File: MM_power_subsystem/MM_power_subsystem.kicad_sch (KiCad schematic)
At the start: 0 parts

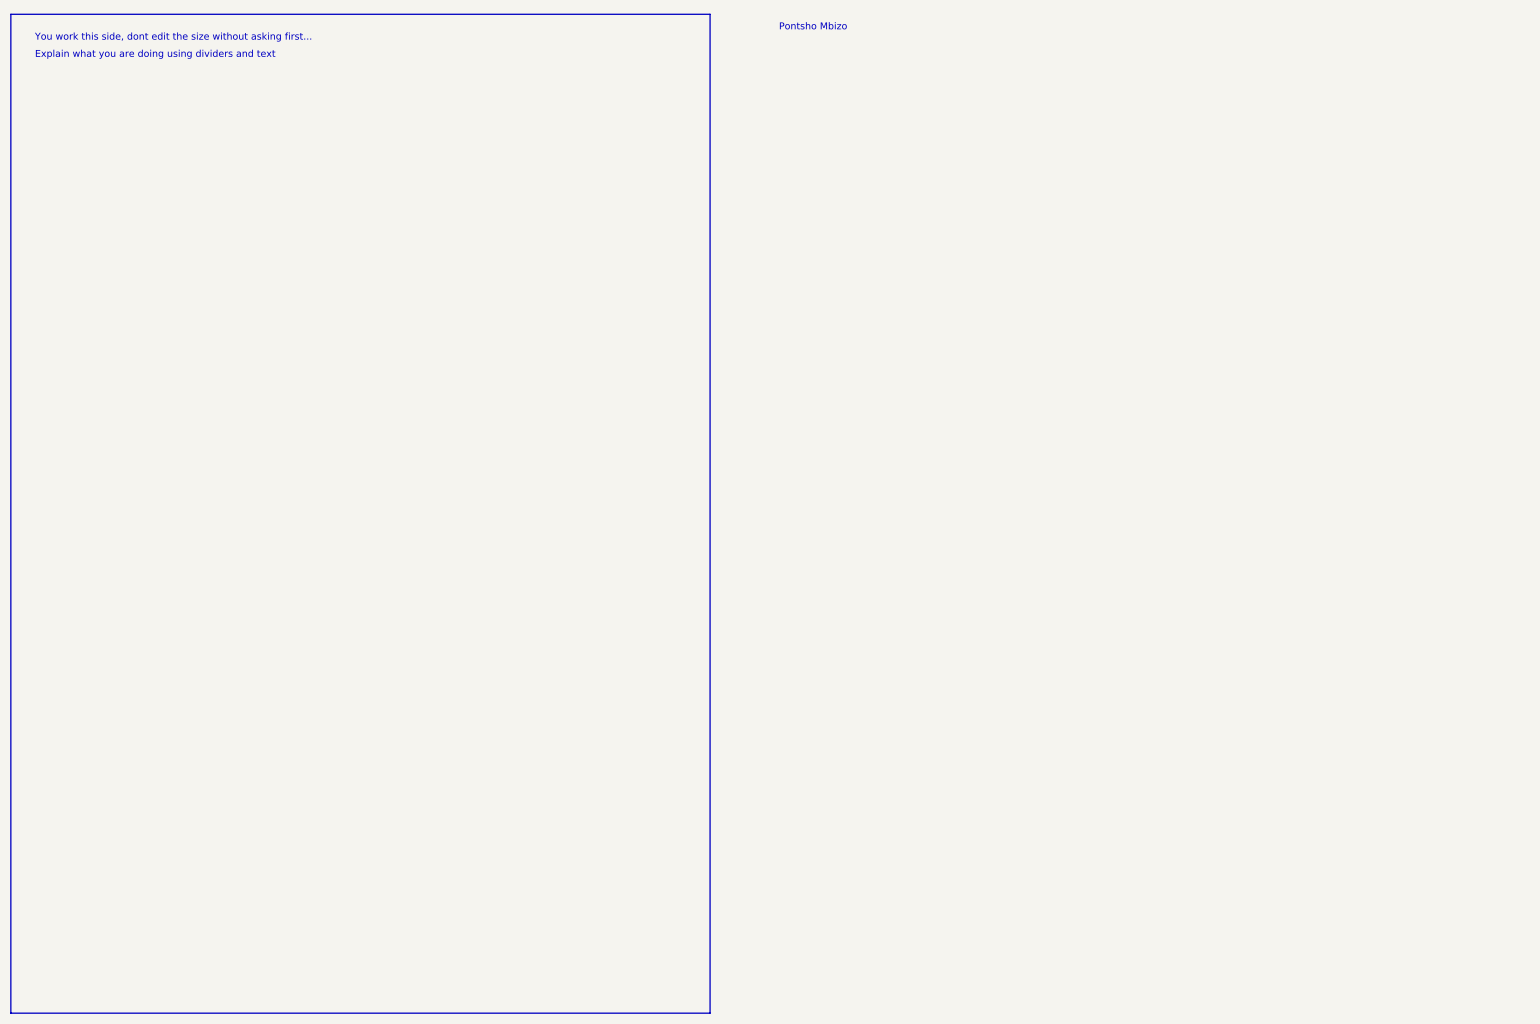
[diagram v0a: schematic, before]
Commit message: Done with the first version of my subsub systems.
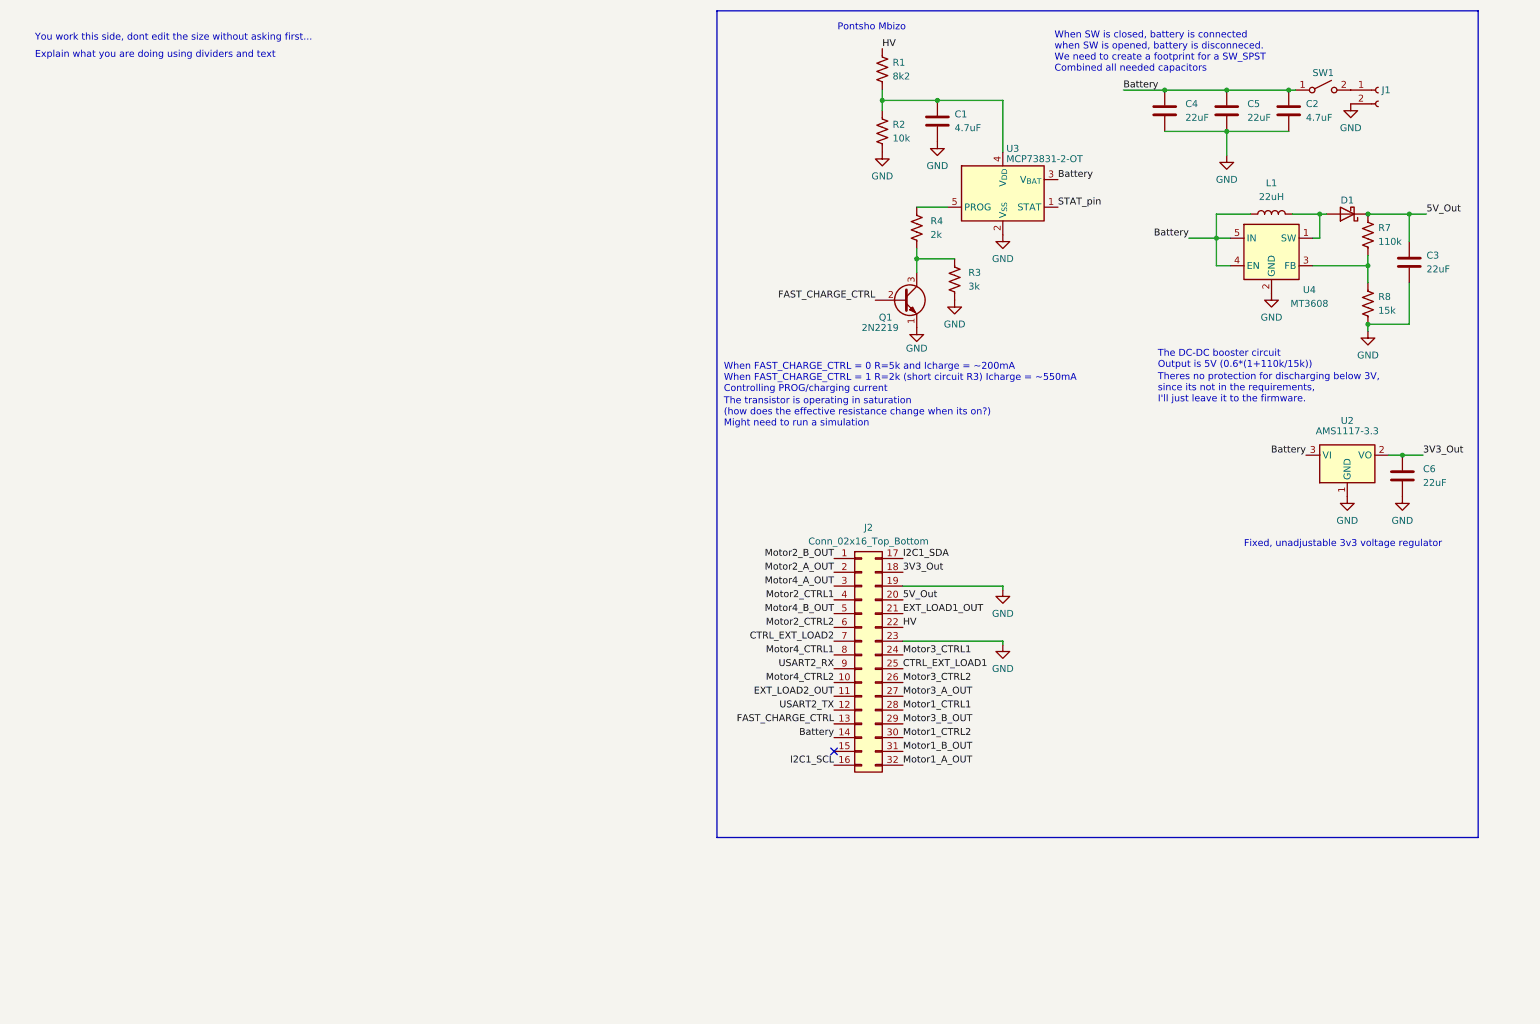
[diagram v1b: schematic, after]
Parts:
- added C1, C2: 4.7uF, symbol Device:C
- added C3, C4, C5, C6: 22uF, symbol Device:C
- added D1: 1N5819, Diode_THT:D_DO-41_SOD81_P10.16mm_Horizontal, symbol Diode:1N5819
- added J1: Conn_01x02_Socket, symbol Connector:Conn_01x02_Socket
- added J2: Conn_02x16_Top_Bottom, Connector_PinHeader_2.54mm:PinHeader_2x16_P2.54mm_Vertical, symbol Connector_Generic:Conn_02x16_Top_Bottom
- added L1: 22uH, symbol Device:L
- added Q1: 2N2219, Package_TO_SOT_THT:TO-39-3, symbol Transistor_BJT:2N2219
- added R1: 8k2, symbol Device:R_US
- added R2: 10k, symbol Device:R_US
- added R3: 3k, symbol Device:R_US
- added R4: 2k, symbol Device:R_US
- added R7: 110k, symbol Device:R_US
- added R8: 15k, symbol Device:R_US
- added SW1: SW_SPST, symbol Switch:SW_SPST
- added U2: AMS1117-3.3, Package_TO_SOT_SMD:SOT-223-3_TabPin2, symbol Regulator_Linear:AMS1117-3.3
- added U3: MCP73831-2-OT, Package_TO_SOT_SMD:SOT-23-5, symbol Battery_Management:MCP73831-2-OT
- added U4: MT3608, Package_TO_SOT_SMD:SOT-23-6, symbol Regulator_Switching:MT3608
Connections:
- new net: D1.2 (A), L1.2, U4.1 (SW)
- new net: R7.2, R8.1, U4.3 (FB)
- new net: R4.1, U3.5 (PROG)
- new net: Q1.3 (C), R3.1, R4.2
- new net: C1.1, R1.2, R2.1, U3.4 (V_{DD})
- new net: J1.1 (Pin_1), SW1.2 (B)
- new net 3V3_Out: C6.1, J2.18 (Pin_18), U2.2 (VO)
- new net 5V_Out: C3.1, D1.1 (K), J2.20 (Pin_20), R7.1
- new net Battery: C2.1, C4.1, C5.1, J2.14 (Pin_14), L1.1, SW1.1 (A), U2.3 (VI), U3.3 (V_{BAT}), U4.4 (EN), U4.5 (IN)
- new net CTRL_EXT_LOAD1: J2.25 (Pin_25)
- new net CTRL_EXT_LOAD2: J2.7 (Pin_7)
- new net EXT_LOAD1_OUT: J2.21 (Pin_21)
- new net EXT_LOAD2_OUT: J2.11 (Pin_11)
- new net FAST_CHARGE_CTRL: J2.13 (Pin_13), Q1.2 (B)
- new net GND: C1.2, C2.2, C3.2, C4.2, C5.2, C6.2, J1.2 (Pin_2), J2.19 (Pin_19), J2.23 (Pin_23), Q1.1 (E), R2.2, R3.2, R8.2, U2.1 (GND), U3.2 (V_{SS}), U4.2 (GND)
- new net HV: J2.22 (Pin_22), R1.1
- new net I2C1_SCL: J2.16 (Pin_16)
- new net I2C1_SDA: J2.17 (Pin_17)
- new net Motor1_A_OUT: J2.32 (Pin_32)
- new net Motor1_B_OUT: J2.31 (Pin_31)
- new net Motor1_CTRL1: J2.28 (Pin_28)
- new net Motor1_CTRL2: J2.30 (Pin_30)
- new net Motor2_A_OUT: J2.2 (Pin_2)
- new net Motor2_B_OUT: J2.1 (Pin_1)
- new net Motor2_CTRL1: J2.4 (Pin_4)
- new net Motor2_CTRL2: J2.6 (Pin_6)
- new net Motor3_A_OUT: J2.27 (Pin_27)
- new net Motor3_B_OUT: J2.29 (Pin_29)
- new net Motor3_CTRL1: J2.24 (Pin_24)
- new net Motor3_CTRL2: J2.26 (Pin_26)
- new net Motor4_A_OUT: J2.3 (Pin_3)
- new net Motor4_B_OUT: J2.5 (Pin_5)
- new net Motor4_CTRL1: J2.8 (Pin_8)
- new net Motor4_CTRL2: J2.10 (Pin_10)
- new net STAT_pin: U3.1 (STAT)
- new net USART2_RX: J2.9 (Pin_9)
- new net USART2_TX: J2.12 (Pin_12)
- no-connect marks 0 -> 1
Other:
- note added: "Fixed, unadjustable 3v3 voltage regulator"
- note added: "The DC-DC booster circuit Output is 5V (0.6*(1+110k/15k))"
- note added: "The transistor is operating in saturation (how does the effective resistance change when its on?) Might need to run a simulation"
- note added: "Theres no protection for discharging below 3V, since its not in the requirements, I'll just leave it to the firmware."
- note added: "When FAST_CHARGE_CTRL = 0 R=5k and Icharge = ~200mA When FAST_CHARGE_CTRL = 1 R=2k (short circuit R3) Icharge = ~550mA Controlling PROG/charging current"
- note added: "When SW is closed, battery is connected when SW is opened, battery is disconneced. We need to create a footprint for a SW_SPST Combined all needed capacitors"

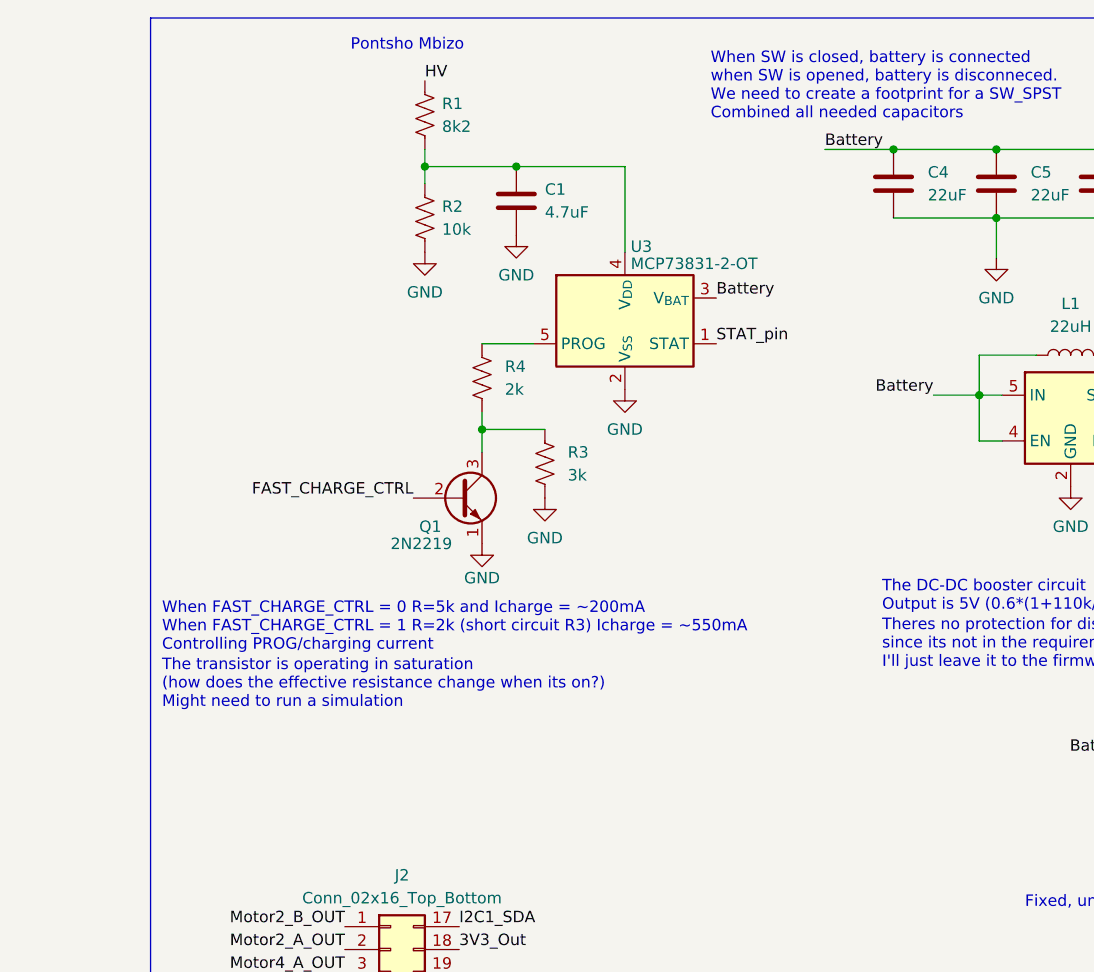
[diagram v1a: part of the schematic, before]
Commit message: annotated
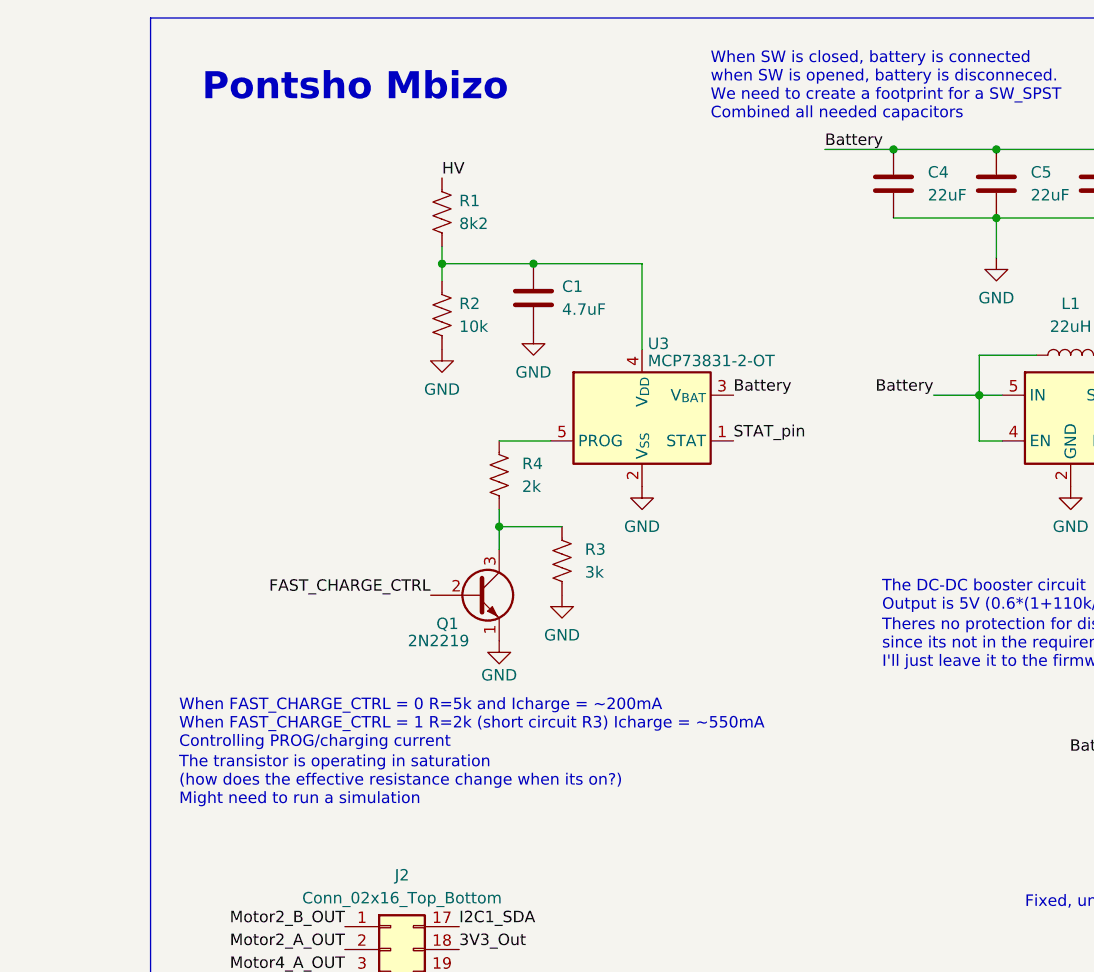
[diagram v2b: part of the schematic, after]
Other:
- moved on the sheet: C1, Q1, R1, R2, R3, R4, U3
